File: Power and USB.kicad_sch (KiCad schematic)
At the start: 11 parts, among them IC4 USBLC6-2SC6, J6 USB4085-GF-A

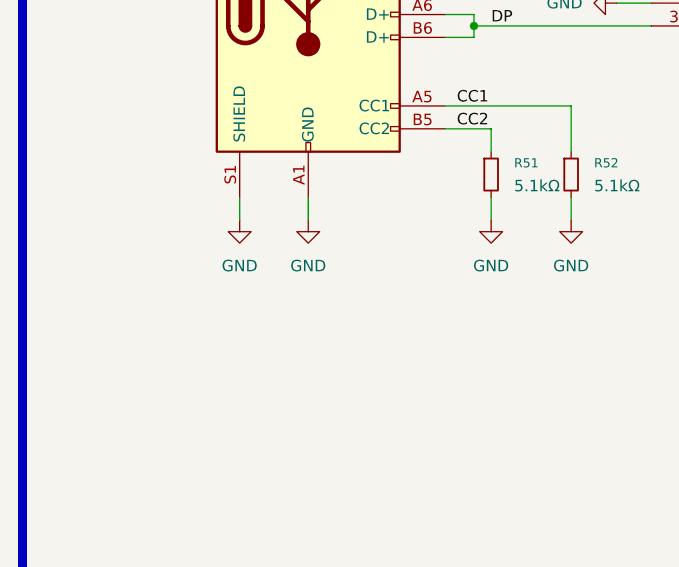
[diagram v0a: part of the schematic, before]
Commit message: fixing drc, generation production files test
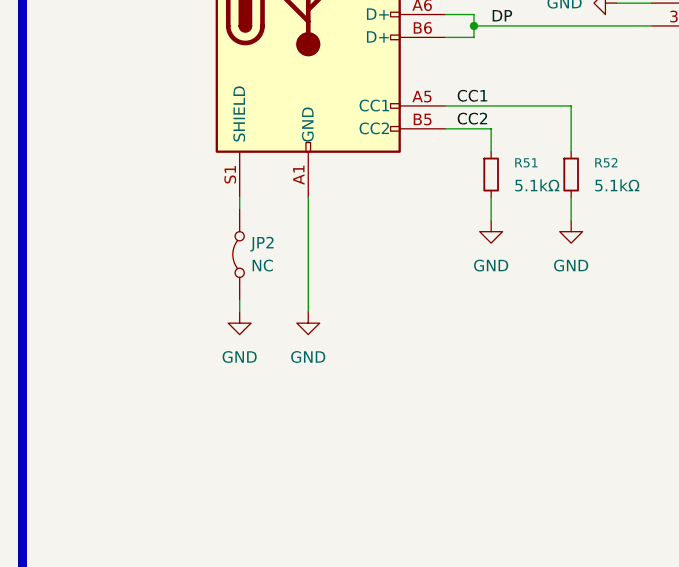
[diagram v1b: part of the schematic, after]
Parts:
- added JP2: NC, Jumper:SolderJumper-2_P1.3mm_Open_TrianglePad1.0x1.5mm, symbol 0_modules:Jumper_2_Bridged
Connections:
- net GND: now also JP2.1 (A); no longer J6.S1 (SHIELD)
- new net: J6.S1 (SHIELD), JP2.2 (B)
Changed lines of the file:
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@@
+		)
+	)
+	(wire
+		(pts
+			(xy 87.63 118.11) (xy 87.63 116.84)
+		)
+		(stroke
+			(width 0)
+			(type default)
 		)
 	)
@@
 	(wire
 		(pts
+			(xy 95.25 105.41) (xy 95.25 118.11)
+		)
+		(stroke
+			(width 0)
+			(type default)
+		)
+	)
+	(wire
+		(pts
 			(xy 250.19 99.06) (xy 266.7 99.06)
 		)
@@
 	(wire
 		(pts
-			(xy 95.25 105.41) (xy 95.25 107.95)
-		)
-		(stroke
-			(width 0)
-			(type default)
-		)
-	)
-	(wire
-		(pts
-			(xy 87.63 105.41) (xy 87.63 107.95)
-		)
-		(stroke
-			(width 0)
-			(type default)
-		)
-	)
-	(wire
-		(pts
 			(xy 110.49 67.31) (xy 170.18 67.31)
 		)
@@
 		(pts
 			(xy 115.57 97.79) (xy 115.57 100.33)
+		)
+		(stroke
+			(width 0)
+			(type default)
+		)
+	)
+	(wire
+		(pts
+			(xy 87.63 105.41) (xy 87.63 106.68)
 		)
 		(stroke
@@
 	(symbol
 		(lib_id "power:GND")
-		(at 87.63 107.95 0)
+		(at 87.63 118.11 0)
 		(unit 1)
 		(exclude_from_sim no)
@@
 		(fields_autoplaced yes)
 		(property "Reference" "#PWR097"
-			(at 87.63 114.3 0)
+			(at 87.63 124.46 0)
 			(effects
 				(font
@@
 		)
 		(property "Value" "GND"
-			(at 87.63 113.03 0)
+			(at 87.63 123.19 0)
 			(effects
 				(font
@@
 		)
 		(property "Footprint" ""
-			(at 87.63 107.95 0)
+			(at 87.63 118.11 0)
 			(effects
 				(font
@@
 		)
 		(property "Datasheet" ""
-			(at 87.63 107.95 0)
+			(at 87.63 118.11 0)
 			(effects
 				(font
@@
 		)
 		(property "Description" "Power symbol creates a global label with name \"GND\" , ground"
-			(at 87.63 107.95 0)
+			(at 87.63 118.11 0)
 			(effects
 				(font
@@
 	(symbol
 		(lib_id "power:GND")
-		(at 95.25 107.95 0)
+		(at 95.25 118.11 0)
 		(unit 1)
 		(exclude_from_sim no)
@@
 		(fields_autoplaced yes)
 		(property "Reference" "#PWR096"
-			(at 95.25 114.3 0)
+			(at 95.25 124.46 0)
 			(effects
 				(font
@@
 		)
 		(property "Value" "GND"
-			(at 95.25 113.03 0)
+			(at 95.25 123.19 0)
 			(effects
 				(font
@@
 		)
 		(property "Footprint" ""
-			(at 95.25 107.95 0)
+			(at 95.25 118.11 0)
 			(effects
 				(font
@@
 		)
 		(property "Datasheet" ""
-			(at 95.25 107.95 0)
+			(at 95.25 118.11 0)
 			(effects
 				(font
@@
 		)
 		(property "Description" "Power symbol creates a global label with name \"GND\" , ground"
-			(at 95.25 107.95 0)
+			(at 95.25 118.11 0)
 			(effects
 				(font
@@
 					(unit 1)
 				)
+			)
+		)
+	)
+	(symbol
+		(lib_id "0_modules:Jumper_2_Bridged")
+		(at 87.63 111.76 90)
+		(unit 1)
+		(exclude_from_sim no)
+		(in_bom yes)
+		(on_board yes)
+		(dnp no)
+		(fields_autoplaced yes)
+		(property "Reference" "JP2"
+			(at 88.9 110.49 90)
+			(effects
+				(font
+					(size 1.27 1.27)
+				)
+				(justify right)
+			)
+		)
+		(property "Value" "NC"
+			(at 88.9 113.03 90)
+			(effects
+				(font
+					(size 1.27 1.27)
+				)
+				(justify right)
+			)
+		)
+		(property "Footprint" "Jumper:SolderJumper-2_P1.3mm_Open_TrianglePad1.0x1.5mm"
+			(at 87.63 111.76 0)
+			(effects
+				(font
+					(size 1.27 1.27)
+				)
+				(hide yes)
+			)
+		)
+		(property "Datasheet" "~"
+			(at 87.63 111.76 0)
+			(effects
+				(font
+					(size 1.27 1.27)
+				)
+				(hide yes)
+			)
+		)
+		(property "Description" "Jumper, 2-pole, closed/bridged"
+			(at 87.63 111.76 0)
+			(effects
+				(font
+					(size 1.27 1.27)
+				)
+				(hide yes)
+			)
+		)
+		(pin "1"
+		)
+		(pin "2"
+		)
+		(instances
+			(project "transmitter"
+				(path "/0650c7a8-acba-429c-9f8e-eec0baf0bc1c/fede4c36-00cc-4d3d-b71c-5243ba232202/97a2efac-bb12-4130-96cc-5d19fa63b112"
+					(reference "JP2")
+					(unit 1)
+				)
